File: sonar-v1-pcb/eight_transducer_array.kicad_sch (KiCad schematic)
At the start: 22 parts, among them U201 ADS8568SPM

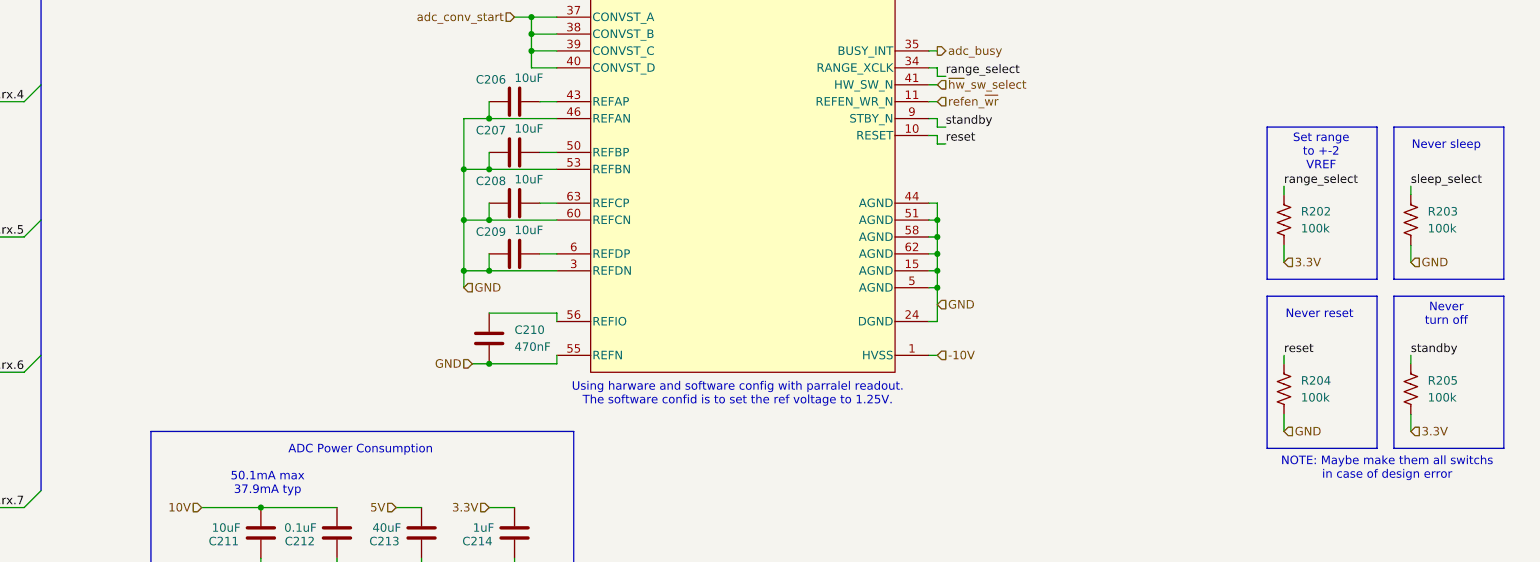
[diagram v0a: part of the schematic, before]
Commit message: formatting lol
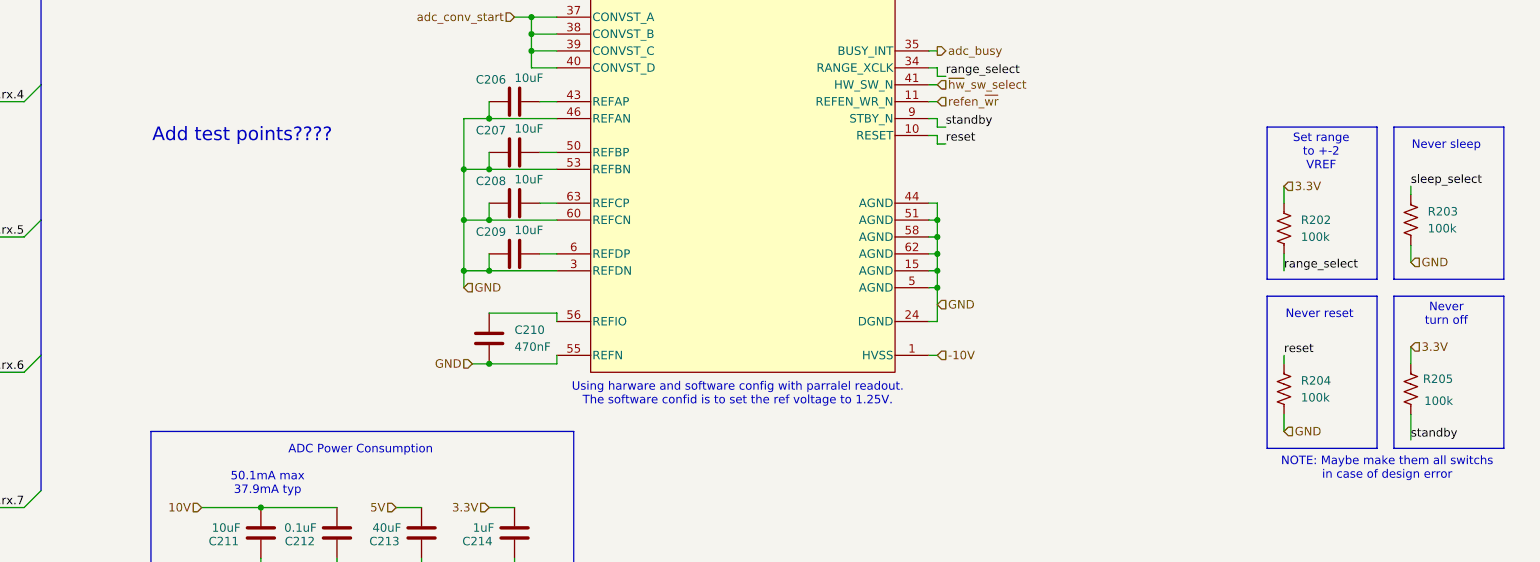
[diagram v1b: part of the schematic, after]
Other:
- note added: "Add test points????"
- moved on the sheet: R202, R205
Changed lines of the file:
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@@
 		)
 	)
+	(text "Add test points????"
+		(exclude_from_sim no)
+		(at 91.186 113.03 0)
+		(effects
+			(font
+				(size 2.032 2.032)
+			)
+		)
+	)
 	(text "208mA max draw on \n+2.5V and -2.5V rails"
 		(exclude_from_sim no)
@@
 	(wire
 		(pts
-			(xy 266.7 154.94) (xy 266.7 157.48)
+			(xy 266.7 147.32) (xy 266.7 144.78)
 		)
 		(stroke
@@
 	(wire
 		(pts
-			(xy 247.65 129.54) (xy 247.65 132.08)
-		)
-		(stroke
-			(width 0)
-			(type default)
-		)
-	)
-	(wire
-		(pts
 			(xy 135.89 34.29) (xy 138.43 34.29)
 		)
@@
 	(wire
 		(pts
+			(xy 247.65 120.65) (xy 247.65 123.19)
+		)
+		(stroke
+			(width 0)
+			(type default)
+		)
+	)
+	(wire
+		(pts
 			(xy 124.46 118.11) (xy 128.27 118.11)
 		)
@@
 	(wire
 		(pts
-			(xy 194.31 62.23) (xy 222.25 62.23)
+			(xy 247.65 133.35) (xy 247.65 130.81)
 		)
 		(stroke
@@
 	(wire
 		(pts
-			(xy 247.65 120.65) (xy 247.65 121.92)
+			(xy 194.31 62.23) (xy 222.25 62.23)
 		)
 		(stroke
@@
 	(wire
 		(pts
-			(xy 266.7 146.05) (xy 266.7 147.32)
+			(xy 266.7 158.75) (xy 266.7 154.94)
 		)
 		(stroke
@@
 	)
 	(label "standby"
-		(at 266.7 146.05 0)
+		(at 266.7 158.75 0)
 		(effects
 			(font
@@
 	)
 	(label "range_select"
-		(at 247.65 120.65 0)
+		(at 247.65 133.35 0)
 		(effects
 			(font
@@
 	(hierarchical_label "3.3V"
 		(shape input)
-		(at 266.7 157.48 0)
+		(at 266.7 144.78 0)
 		(effects
 			(font
@@
 	(hierarchical_label "3.3V"
 		(shape input)
-		(at 247.65 132.08 0)
+		(at 247.65 120.65 0)
 		(effects
 			(font
@@
 	(symbol
 		(lib_id "Device:R_US")
-		(at 266.7 151.13 0)
+		(at 266.7 151.13 180)
 		(unit 1)
 		(exclude_from_sim no)
@@
 		(on_board yes)
 		(dnp no)
-		(fields_autoplaced yes)
 		(property "Reference" "R205"
-			(at 269.24 149.8599 0)
+			(at 273.05 149.606 0)
 			(effects
 				(font
@@
 		)
 		(property "Value" "100k"
-			(at 269.24 152.3999 0)
+			(at 273.05 152.908 0)
 			(effects
 				(font
@@
 		)
 		(property "Footprint" "Resistor_SMD:R_0402_1005Metric"
-			(at 267.716 151.384 90)
+			(at 265.684 150.876 90)
 			(effects
 				(font
@@
 	(symbol
 		(lib_id "Device:R_US")
-		(at 247.65 125.73 0)
+		(at 247.65 127 180)
 		(unit 1)
 		(exclude_from_sim no)
@@
 		(fields_autoplaced yes)
 		(property "Reference" "R202"
-			(at 250.19 124.4599 0)
+			(at 250.19 125.7299 0)
 			(effects
 				(font
 					(size 1.27 1.27)
 				)
-				(justify left)
+				(justify right)
 			)
 		)
 		(property "Value" "100k"
-			(at 250.19 126.9999 0)
+			(at 250.19 128.2699 0)
 			(effects
 				(font
 					(size 1.27 1.27)
 				)
-				(justify left)
+				(justify right)
 			)
 		)
 		(property "Footprint" "Resistor_SMD:R_0402_1005Metric"
-			(at 248.666 125.984 90)
+			(at 246.634 126.746 90)
 			(effects
 				(font
@@
 		)
 		(property "Datasheet" "~"
-			(at 247.65 125.73 0)
+			(at 247.65 127 0)
 			(effects
 				(font
@@
 		)
 		(property "Description" "Resistor, US symbol"
-			(at 247.65 125.73 0)
+			(at 247.65 127 0)
 			(effects
 				(font
@@
 		)
 		(fill
-			(color 0 0 0 0.0000)
+			(color 194 194 194 1.0000)
 		)
 		(property "Sheetname" "rx_amp_7"
@@
 		)
 		(fill
-			(color 0 0 0 0.0000)
+			(color 194 194 194 1.0000)
 		)
 		(property "Sheetname" "rx_amp_2"
@@
 		)
 		(fill
-			(color 0 0 0 0.0000)
+			(color 194 194 194 1.0000)
 		)
 		(property "Sheetname" "rx_amp_1"
@@
 		)
 		(fill
-			(color 0 0 0 0.0000)
+			(color 194 194 194 1.0000)
 		)
 		(property "Sheetname" "rx_amp_5"
@@
 		)
 		(fill
-			(color 0 0 0 0.0000)
+			(color 194 194 194 1.0000)
 		)
 		(property "Sheetname" "rx_amp_0"
@@
 		)
 		(fill
-			(color 0 0 0 0.0000)
+			(color 194 194 194 1.0000)
 		)
 		(property "Sheetname" "rx_amp_4"
@@
 		)
 		(fill
-			(color 0 0 0 0.0000)
+			(color 194 194 194 1.0000)
 		)
 		(property "Sheetname" "rx_amp_3"
@@
 		)
 		(fill
-			(color 0 0 0 0.0000)
+			(color 194 194 194 1.0000)
 		)
 		(property "Sheetname" "rx_amp_6"
